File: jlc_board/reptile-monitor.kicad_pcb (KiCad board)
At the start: 4 copper layers, 38.1 x 84.6 mm, 45 parts, among them J1 USB_C_Receptacle_USB2.0, J2 AC_IN, J3 Conn_01x08, J7 LOAD1, J8 LOAD2, K1 ALDP105W, K2 ALDP105W, SW1 RST, SW2 BOOT, U1 ESP32-S2-WROVER, U2 TPS2112PW, U3 AP2112K-3.3, U4 MDC3105LT1G, U5 MDC3105LT1G, Y1 32.768KHz 12.5p

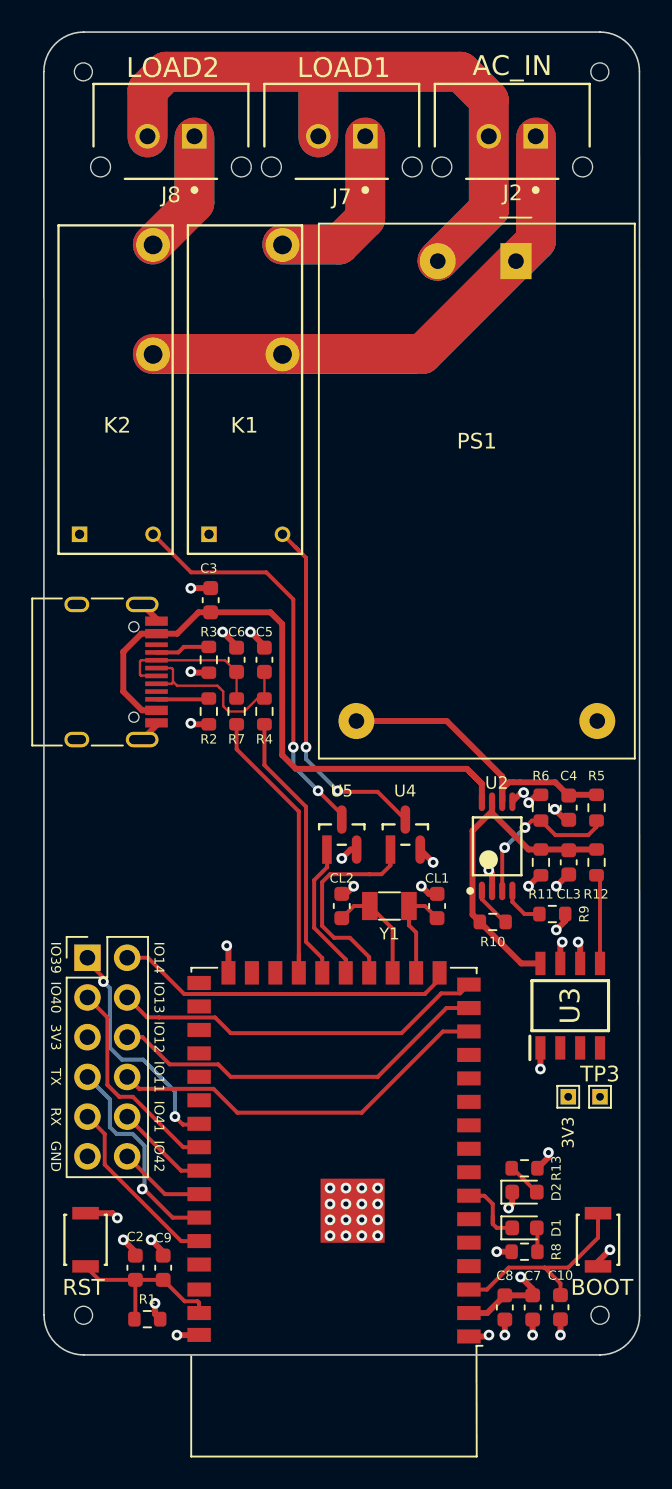
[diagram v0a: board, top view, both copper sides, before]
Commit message: rev2
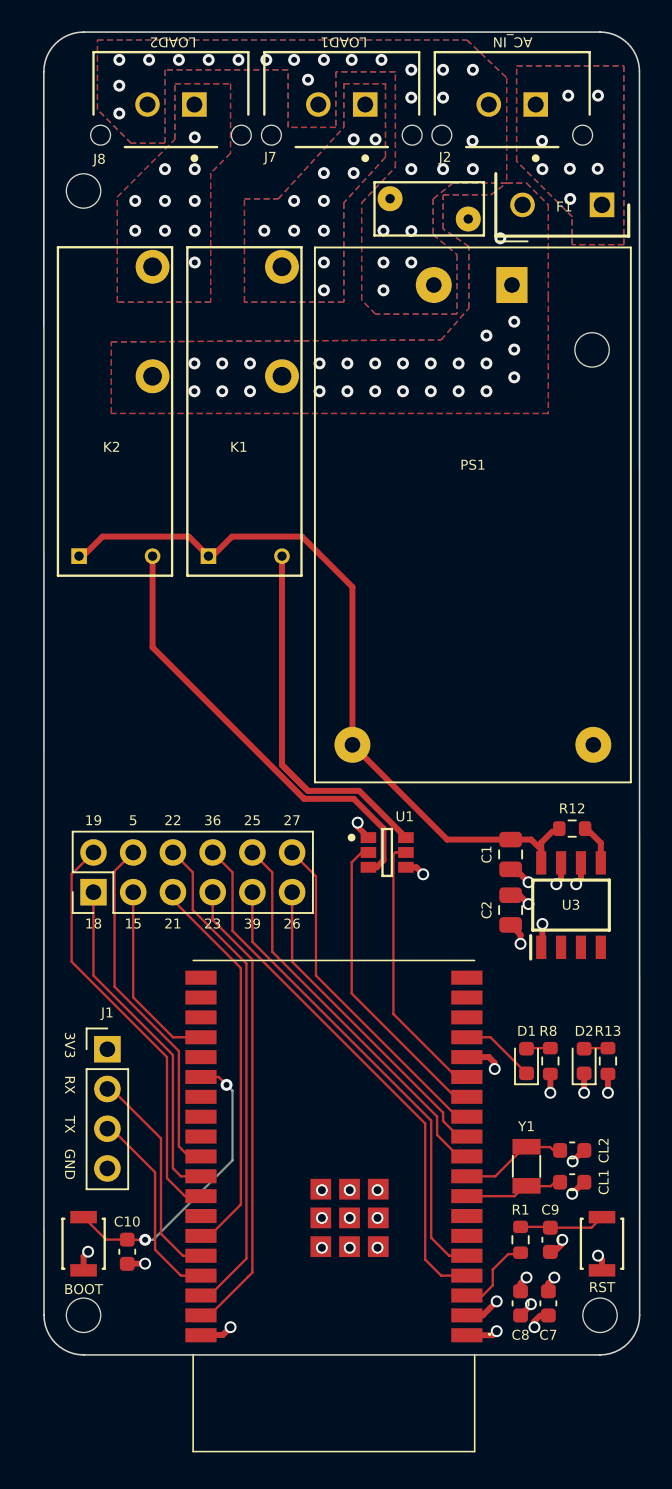
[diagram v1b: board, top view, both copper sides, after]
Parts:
- removed C3, C4: 0.1u, Capacitor_SMD:C_0603_1608Metric
- removed C5, C6: 20p, Capacitor_SMD:C_0603_1608Metric
- removed CL3: 10u, Capacitor_SMD:C_0603_1608Metric
- removed R10, R11: 10k, Resistor_SMD:R_0603_1608Metric
- removed R2, R3: 5.1k, Resistor_SMD:R_0603_1608Metric
- removed R4, R7: 22r, Resistor_SMD:R_0603_1608Metric
- removed R5: 2.2k, Resistor_SMD:R_0603_1608Metric
- removed R6: 1k, Resistor_SMD:R_0603_1608Metric
- removed R9: 500r, Resistor_SMD:R_0603_1608Metric
- removed TP1: 3V3, TestPoint:TestPoint_THTPad_1.0x1.0mm_Drill0.5mm
- removed TP3: GND, TestPoint:TestPoint_THTPad_1.0x1.0mm_Drill0.5mm
- removed U2: TPS2112PW, Reptile_Monitor:Texas_Instruments-TPS2112PW
- removed U4, U5: MDC3105LT1G, Reptile_Monitor:ON_Semiconductor-318-08-01_2018-AS
- added C1: 1u, Capacitor_SMD:C_0805_2012Metric, F.Cu at (161.2, 87.4)
- added F1: 39215000000, SamacSys_Parts:TO508P400X850X850-2P, F.Cu at (167.0, 45.8)
- added IC1: ESP32-WROVER-E_M213EH6464PH3Q0_, SamacSys_Parts:ESP32WROVEREM213EH6464PH3Q0, F.Cu at (149.9, 109.9)
- added REF1: MountingHole_2.2mm_M2, MountingHole:MountingHole_2.2mm_M2, F.Cu at (166.4, 55.1)
- added REF1: MountingHole_2.2mm_M2, MountingHole:MountingHole_2.2mm_M2, F.Cu at (133.9, 45.0)
- added REF2: MountingHole_2.2mm_M2, MountingHole:MountingHole_2.2mm_M2, F.Cu at (133.9, 116.8)
- added REF3: MountingHole_2.2mm_M2, MountingHole:MountingHole_2.2mm_M2, F.Cu at (166.9, 116.8)
- added RV1: Varistor, Varistor:RV_Disc_D7mm_W3.4mm_P5mm, F.Cu at (153.5, 45.5)
- added WAFFLE: LOGO, LOGO, B.Cu at (151.3, 105.7)
- added WESLEY: LOGO, LOGO, B.Cu at (142.0, 78.1)
- added svg2mod: G***, svg2mod, B.Cu at (159.8, 74.8)
- added svg2mod: G***, svg2mod, B.Cu at (154.8, 85.2)
- C2: value 0.1u -> 1u; footprint Capacitor_SMD:C_0603_1608Metric -> Capacitor_SMD:C_0805_2012Metric
- J1: value USB_C_Receptacle_USB2.0 -> UART; footprint Reptile_Monitor:USB_C_Receptacle_HRO_TYPE-C-31-M-12 -> Connector_PinHeader_2.54mm:PinHeader_1x04_P2.54mm_Vertical
- U1: value ESP32-S2-WROVER -> NUD3105DMT1G; footprint RF_Module:ESP32-S2-WROVER -> reptile-monitor:ON_Semi-318F-0-0-0
- Y1: footprint Reptile_Monitor:Crystal_SMD_3215-2Pin_3.2x1.5mm -> reptile-monitor:Crystal_SMD_3215-2Pin_3.2x1.5mm
- moved C2 33.1 mm to (161.2, 90.9), turned to -90 degrees
- moved SW1 33.0 mm to (167.0, 112.3), turned to -90 degrees
- moved SW2 32.9 mm to (133.9, 112.3)
- moved C10 27.9 mm to (136.7, 112.8)
- moved C9 24.8 mm to (163.7, 112.0), turned to -90 degrees
- moved R1 24.4 mm to (161.8, 112.0), turned to 90 degrees
- moved J1 24.1 mm to (135.4, 99.8), turned to 0 degrees
- moved CL2 21.5 mm to (165.1, 106.3), turned to 0 degrees
- moved CL1 19.7 mm to (165.1, 108.3), turned to 0 degrees
- moved U1 19.5 mm to (153.3, 87.2), turned to 0 degrees
- moved Y1 18.8 mm to (162.2, 107.3), turned to 90 degrees
- moved R8 12.3 mm to (163.7, 100.6), turned to -90 degrees
- moved D1 10.7 mm to (162.2, 100.6), turned to 90 degrees
- moved D2 9.21 mm to (165.9, 100.6), turned to 90 degrees
- moved R13 8.69 mm to (167.4, 100.6), turned to 90 degrees
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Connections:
- net Net-(R12-Pad1) renamed /PWR_EN
- C2 pad 1: /EN -> GND
- C2 pad 2: GND -> +3V3
- C9 pad 1: /EN -> Net-(C9-Pad1)
- CL1 pad 1: /IO15 -> Net-(CL1-Pad1)
- CL2 pad 1: /IO16 -> Net-(CL2-Pad1)
- D1 pad 1: Net-(D1-Pad1) -> /IO13
- J3 pad 1: /IO39 -> /IO18
- J3 pad 10: /IO41 -> /IO25
- J3 pad 11: GND -> /IO26
- J3 pad 12: /IO42 -> /IO27
- J3 pad 2: /IO14 -> /IO19
- J3 pad 3: /IO40 -> /IO15
- J3 pad 4: /IO13 -> /IO5
- J3 pad 5: +3V3 -> /IO21
- J3 pad 6: /IO12 -> /IO22
- J3 pad 7: /TXD0 -> /IO23
- J3 pad 8: /IO11 -> /IO36
- J3 pad 9: /RXD0 -> /IO39
- K1 pad 1: GND -> +5V
- K1 pad 3: /AC_L -> /FUSED_AC_L
- K1 pad 4: Net-(K1-Pad4) -> /RLY1
- K2 pad 1: GND -> +5V
- K2 pad 3: /AC_L -> /FUSED_AC_L
- K2 pad 4: Net-(K2-Pad4) -> /RLY2
- PS1 pad 1: /AC_L -> /FUSED_AC_L
- PS1 pad 4: VCC -> +5V
- R1 pad 1: +3V3 -> /EN
- R1 pad 2: /EN -> Net-(C9-Pad1)
- SW1 pad 1: /EN -> Net-(C9-Pad1)
- U1 pad 2: +3V3 -> /IO14
- U1 pad 3: /IO0 -> /RLY2
- U1 pad 4: (no net) -> GND
- U1 pad 5: (no net) -> /IO12
- U1 pad 6: (no net) -> /RLY1
- U3 pad 2: (no net) -> unconnected-(U3-Pad2)
- U3 pad 3: (no net) -> unconnected-(U3-Pad3)
- U3 pad 4: (no net) -> unconnected-(U3-Pad4)
- Y1 pad 1: /IO16 -> Net-(CL2-Pad1)
- Y1 pad 2: /IO15 -> Net-(CL1-Pad1)
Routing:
- net /AC_N: track 280.0 -> 0.00 mm, vias 0 -> 27
- net /AC_L: track 204.7 -> 0.00 mm, vias 0 -> 7
- net /LOAD1: track 67.1 -> 0.00 mm, vias 0 -> 11
- net /LOAD2: track 47.7 -> 0.00 mm, vias 0 -> 10
- net VBUS: track 40.9 -> 0.00 mm
- net /IO36: track 0.00 -> 34.7 mm
- net /IO22: track 0.00 -> 31.8 mm
- net /IO23: track 0.00 -> 29.9 mm
- net /RLY2: track 0.00 -> 28.3 mm
- net /IO19: track 0.00 -> 26.6 mm
- net +5V: track 22.0 -> 48.1 mm
- net Net-(K2-Pad4): track 26.1 -> 0.00 mm, vias 2 -> 0
- net /IO25: track 0.00 -> 25.4 mm
- net /IO21: track 0.00 -> 25.2 mm
- net /RLY1: track 0.00 -> 25.1 mm
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- added copper zone on B.Cu, net /AC_L
- added copper zone on F.Cu, net /AC_L
- added copper zone on In1.Cu, net /AC_L
- added copper zone on In2.Cu, net /AC_L
- added copper zone on B.Cu, net /AC_N
- added copper zone on F.Cu, net /AC_N
- added copper zone on In1.Cu, net /AC_N
- added copper zone on In2.Cu, net /AC_N
- added copper zone on B.Cu, net /FUSED_AC_L
- added copper zone on F.Cu, net /FUSED_AC_L
- added copper zone on In1.Cu, net /FUSED_AC_L
- added copper zone on In2.Cu, net /FUSED_AC_L
- added copper zone on B.Cu, net /LOAD1
- added copper zone on F.Cu, net /LOAD1
- added copper zone on In1.Cu, net /LOAD1
- added copper zone on In2.Cu, net /LOAD1
- added copper zone on B.Cu, net /LOAD2
- added copper zone on F.Cu, net /LOAD2
- added copper zone on In1.Cu, net /LOAD2
- added copper zone on In2.Cu, net /LOAD2
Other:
- outline, holes or cut-outs redrawn
- board text added: "15"
- board text added: "18"
- board text added: "19"
- board text added: "21"
- board text added: "22"
- board text added: "23"
- board text added: "25"
- board text added: "26"
- board text added: "27"
- board text added: "36"
- board text added: "39"
- board text added: "5"
- board text added: "Rev 2 April 2021"
- board text removed: "ESP32-S2 Reptile Monitor Mike Pleimann Rev 2 April 2021"
- board text removed: "IO11"
- board text removed: "IO12"
- board text removed: "IO13"
- board text removed: "IO14"
- board text removed: "IO39"
- board text removed: "IO40"
- board text removed: "IO41"
- board text removed: "IO42"
